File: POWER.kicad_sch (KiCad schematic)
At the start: 22 parts, among them J100 VCC INPUT, J101 SWITCH ON/OFF, J102 FAN VOLTAGE, Q100 WST4045, U1 AMS1117-3.3, U100 LM2596S-5

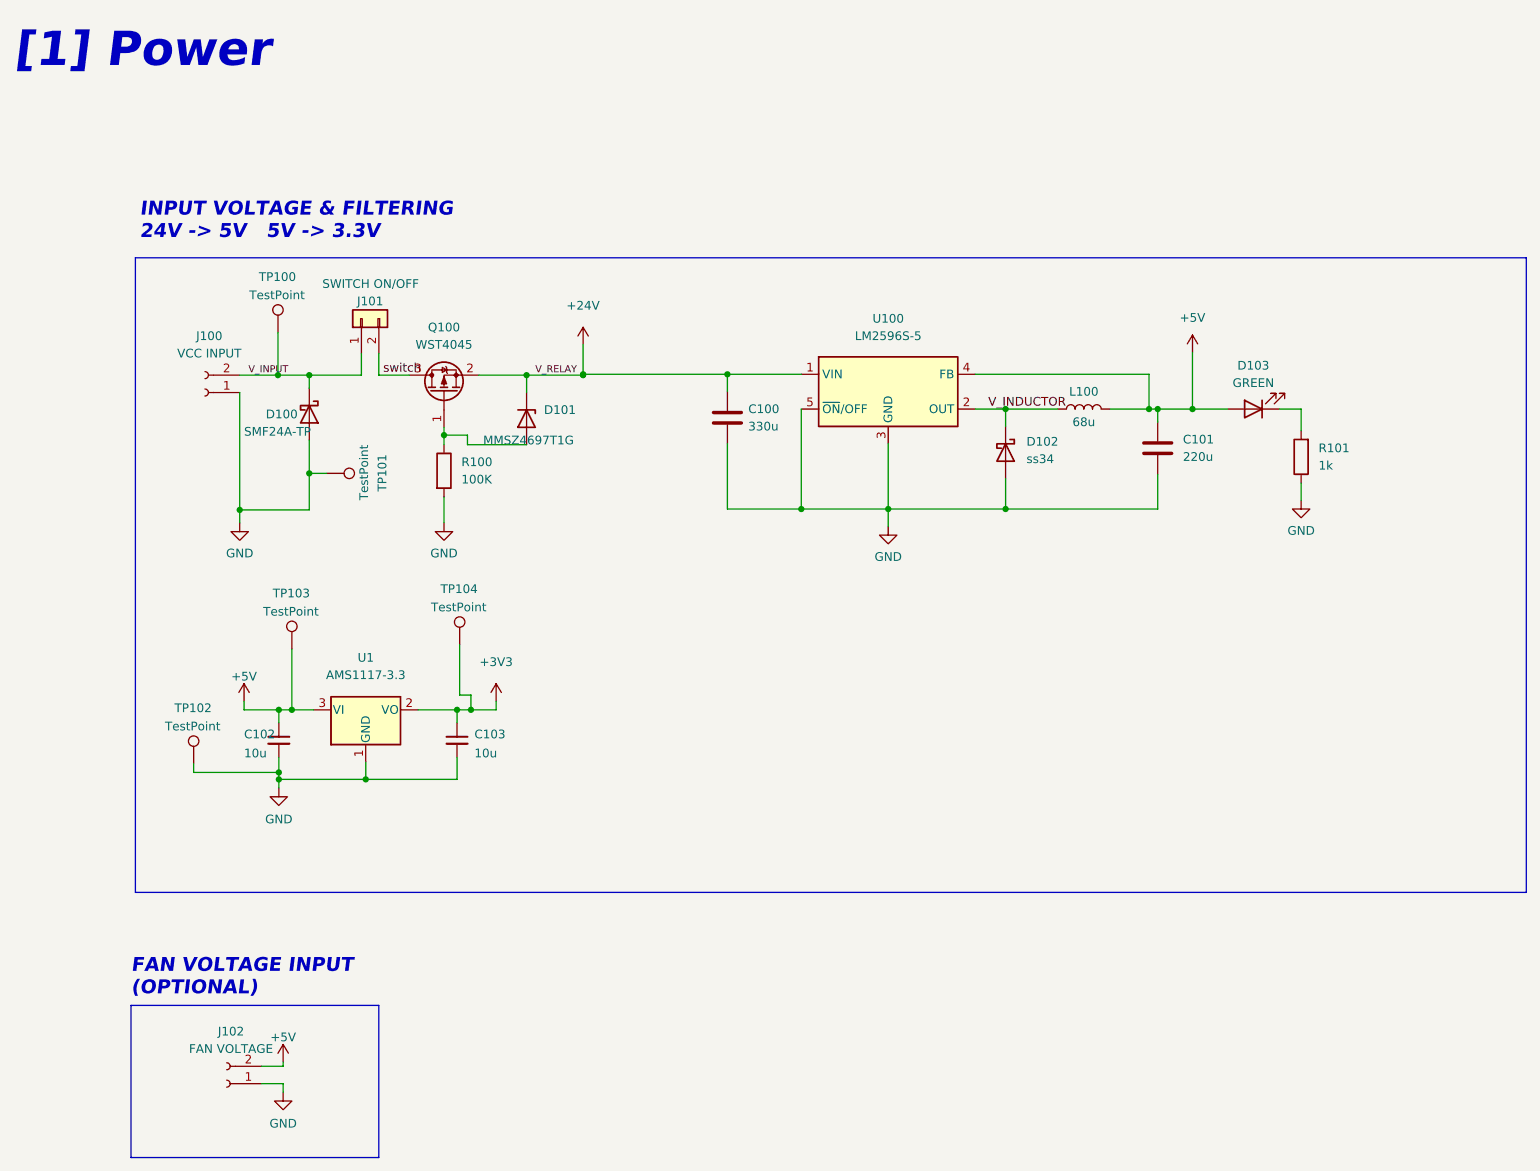
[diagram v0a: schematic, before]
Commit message: version validada
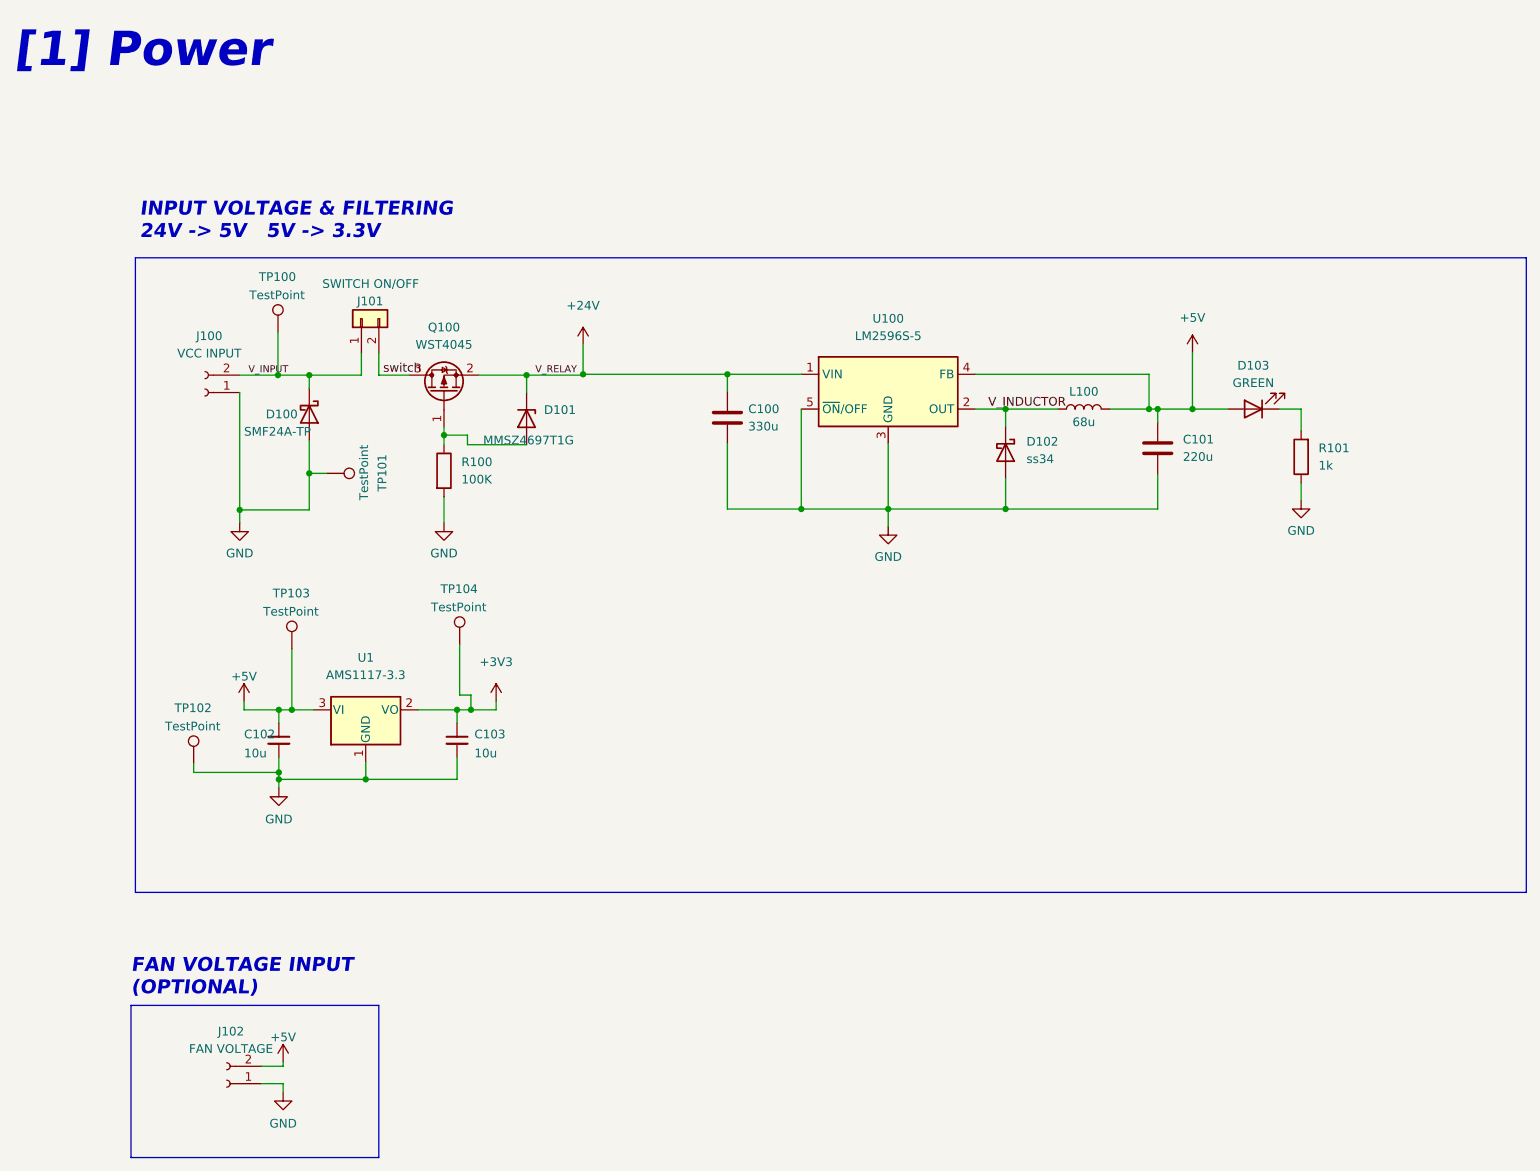
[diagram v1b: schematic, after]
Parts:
- J101: footprint Connector_PinHeader_2.54mm:PinHeader_1x02_P2.54mm_Vertical -> B2B-XH-A:JST_B2B-XH-A_LF__SN_
- L100: footprint Jose_:SMD_12.3X12.3mm -> Inductor_SMD_Jose:L_12.3x12.3
